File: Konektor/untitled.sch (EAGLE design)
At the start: 10 parts, among them J1 RJ45-8N-B, J2 RJ45-8N-B, X1 MSTBA2, X2 MSTBA5, X3 MSTBA5, X6 MSTBA2, X7 C-GRID-02-70543, X8 MSTBA2

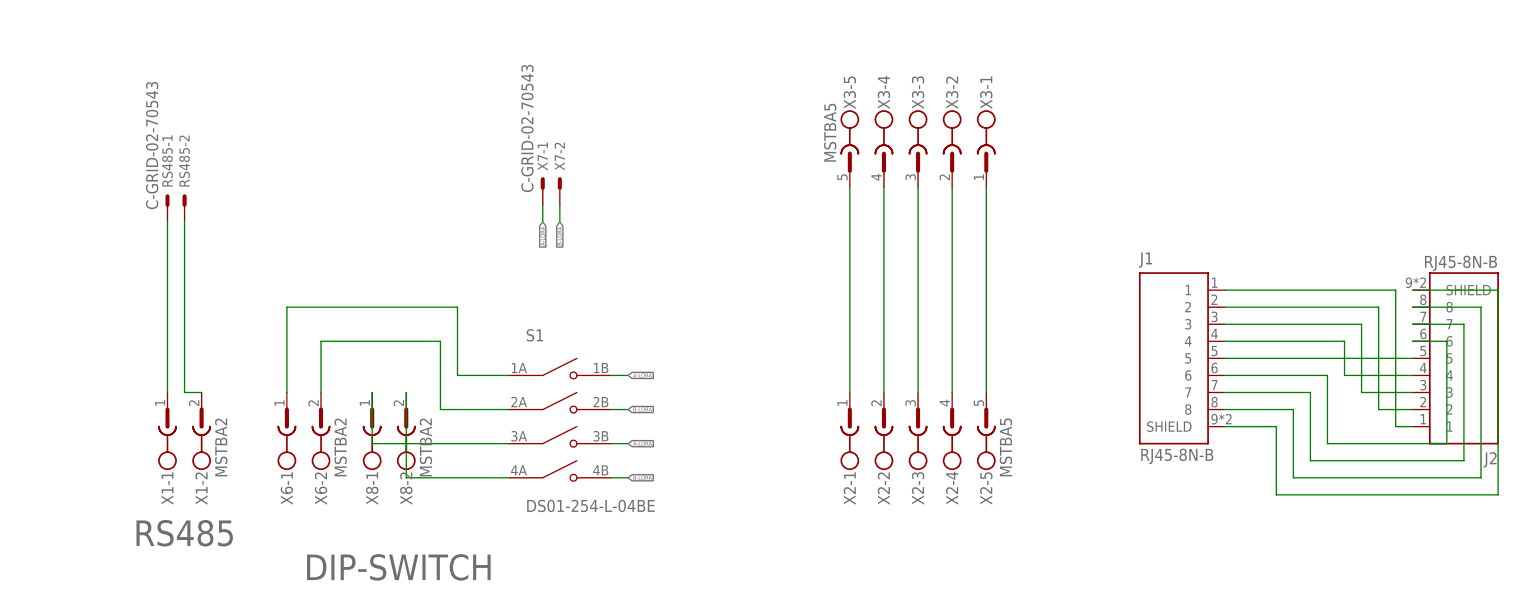
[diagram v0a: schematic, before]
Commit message: 3 PCB done
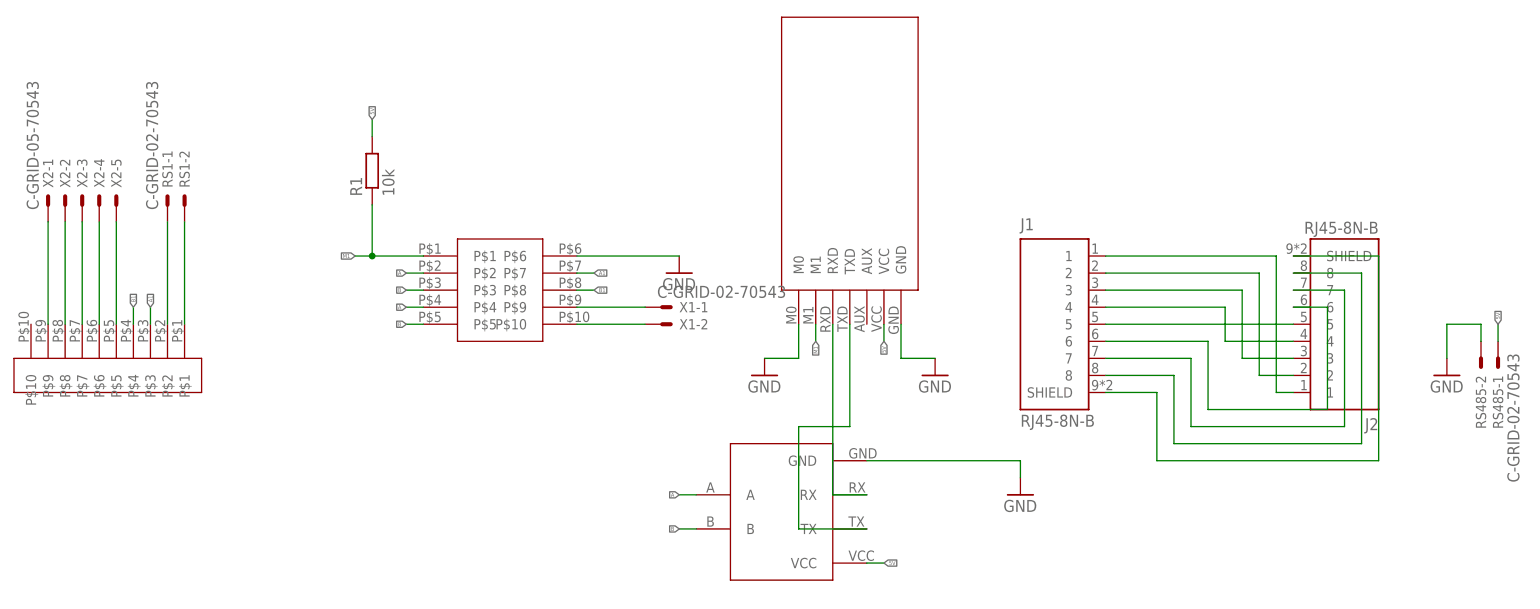
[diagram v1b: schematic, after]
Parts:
- removed S1: DS01-254-L-04BE, DS01-254-L-04BE:DS01-254-L-04BE
- removed X3: MSTBA5, con-phoenix-508:MSTBA5
- removed X6, X8: MSTBA2, con-phoenix-508:MSTBA2
- removed X7: C-GRID-02-70543, con-molex:C-GRID-02-70543
- added DP-05RP1: (no value), DP-05RP:DP-05RP
- added EBYTEE220-900T22D1: (no value), EByte E220-900T22D:EBYTEE220-900T22D
- added KONEKTOR-3.81-13P1: (no value), KONEKTOR-3.81-13P:KONEKTOR-3.81-13P
- added R1: 10k, rcl:R-EU_R0805
- added RS1: C-GRID-02-70543, con-molex:C-GRID-02-70543
- added TTL-RS1: (no value), TTL-RS485:TTL-RS485
- X1: value MSTBA2 -> C-GRID-02-70543; device con-phoenix-508:MSTBA2 -> con-molex:C-GRID-02-70543
- X2: value MSTBA5 -> C-GRID-05-70543; device con-phoenix-508:MSTBA5 -> con-molex:C-GRID-05-70543
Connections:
- removed net A-LORA: S1.NO1, S1.NO3, X7-1.S
- removed net B-LORA: S1.NO2, S1.NO4, X7-2.S
- new net 5V: EBYTEE220-900T22D1.VCC, R1.2, RS485-1.S, TTL-RS1.VCC
- new net A: DP-05RP1.P$2, DP-05RP1.P$4, TTL-RS1.A
- new net A1: DP-05RP1.P$7, KONEKTOR-3.81-13P1.P$3
- new net B: DP-05RP1.P$3, DP-05RP1.P$5, TTL-RS1.B
- new net B1: DP-05RP1.P$8, KONEKTOR-3.81-13P1.P$4
- new net GND: DP-05RP1.P$6, EBYTEE220-900T22D1.GND, EBYTEE220-900T22D1.M0, RS485-2.S, TTL-RS1.GND
- new net M1: DP-05RP1.P$1, EBYTEE220-900T22D1.M1, R1.1
- net N$1: now also KONEKTOR-3.81-13P1.P$1, RS1-2.S; no longer RS485-1.S, X1-1.1
- net N$15: now also KONEKTOR-3.81-13P1.P$6, X2-4.S; no longer S1.COM1, X6-1.1
- net N$16: now also KONEKTOR-3.81-13P1.P$7, X2-3.S; no longer S1.COM2, X6-2.1
- net N$17: now also KONEKTOR-3.81-13P1.P$8, X2-2.S; no longer S1.COM3, X8-1.1
- net N$18: now also KONEKTOR-3.81-13P1.P$9, X2-1.S; no longer S1.COM4, X8-2.1
- net N$2: now also KONEKTOR-3.81-13P1.P$2, RS1-1.S; no longer RS485-2.S, X1-2.1
- net N$3: now also EBYTEE220-900T22D1.RXD, TTL-RS1.RX; no longer X2-1.1, X3-5.1
- net N$4: now also EBYTEE220-900T22D1.TXD, TTL-RS1.TX; no longer X2-2.1, X3-4.1
- net N$5: now also DP-05RP1.P$9, X1-1.S; no longer X2-3.1, X3-3.1
- net N$6: now also DP-05RP1.P$10, X1-2.S; no longer X2-4.1, X3-2.1
- net N$7: now also KONEKTOR-3.81-13P1.P$5, X2-5.S; no longer X2-5.1, X3-1.1
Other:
- note removed: "DIP-SWITCH"
- note removed: "RS485"
- moved on the sheet: J1, J2, RS485-1, RS485-2
